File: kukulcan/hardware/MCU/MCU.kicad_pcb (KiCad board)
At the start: 4 copper layers, 90.1 x 64.4 mm, 90 parts, among them J1 Barrel_Jack_5V_In, J2 Barrel_Jack_5V_In, J3 USB_C_Receptacle, J4 SMA_GNSS, Q1 AO3401A, U1 TLV1117-33, U2 W25Q256JWEIQ, U3 ESP32-S3R16V, U4 BNO055, U5 NEO-M8N, U6 BMI088, U7 BME280, X1 40MHz, Y1 32.768kHz

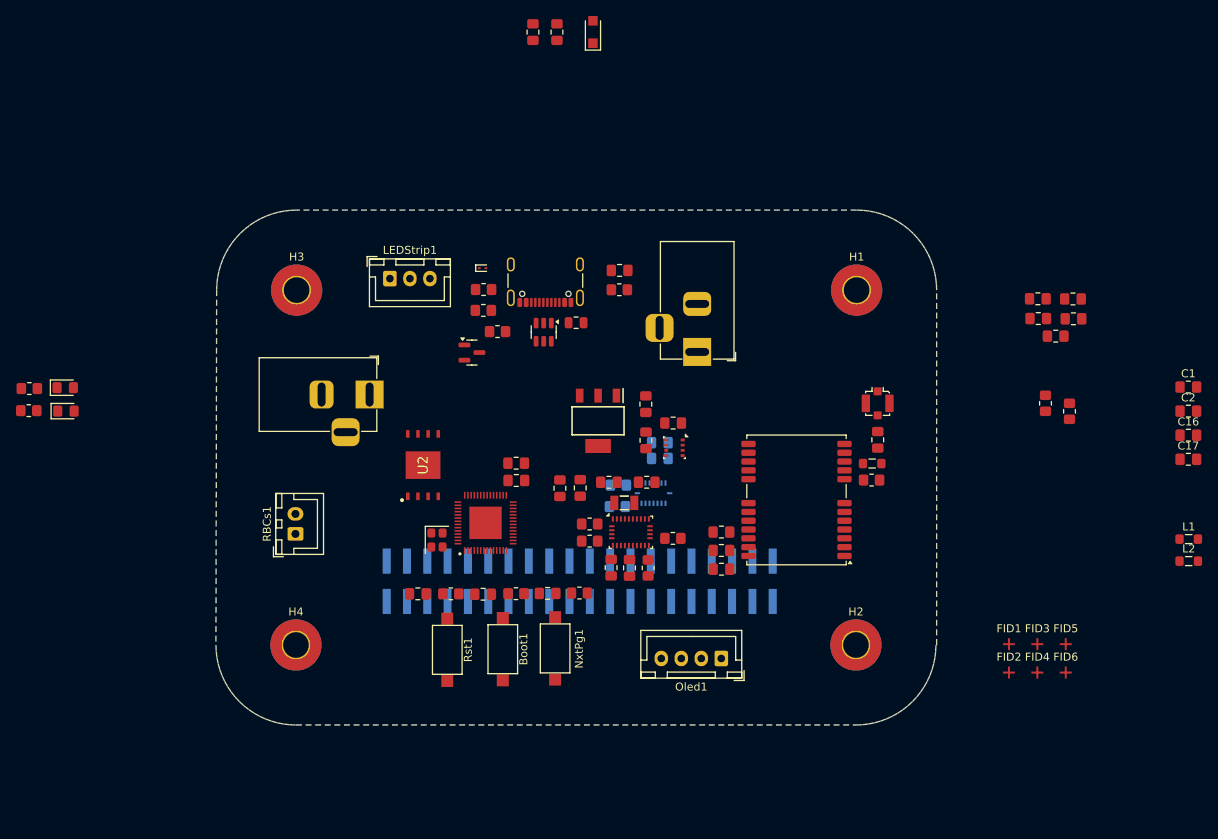
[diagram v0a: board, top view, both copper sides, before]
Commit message: feat(kukulcan): partial final PCB draft, GNSS pending
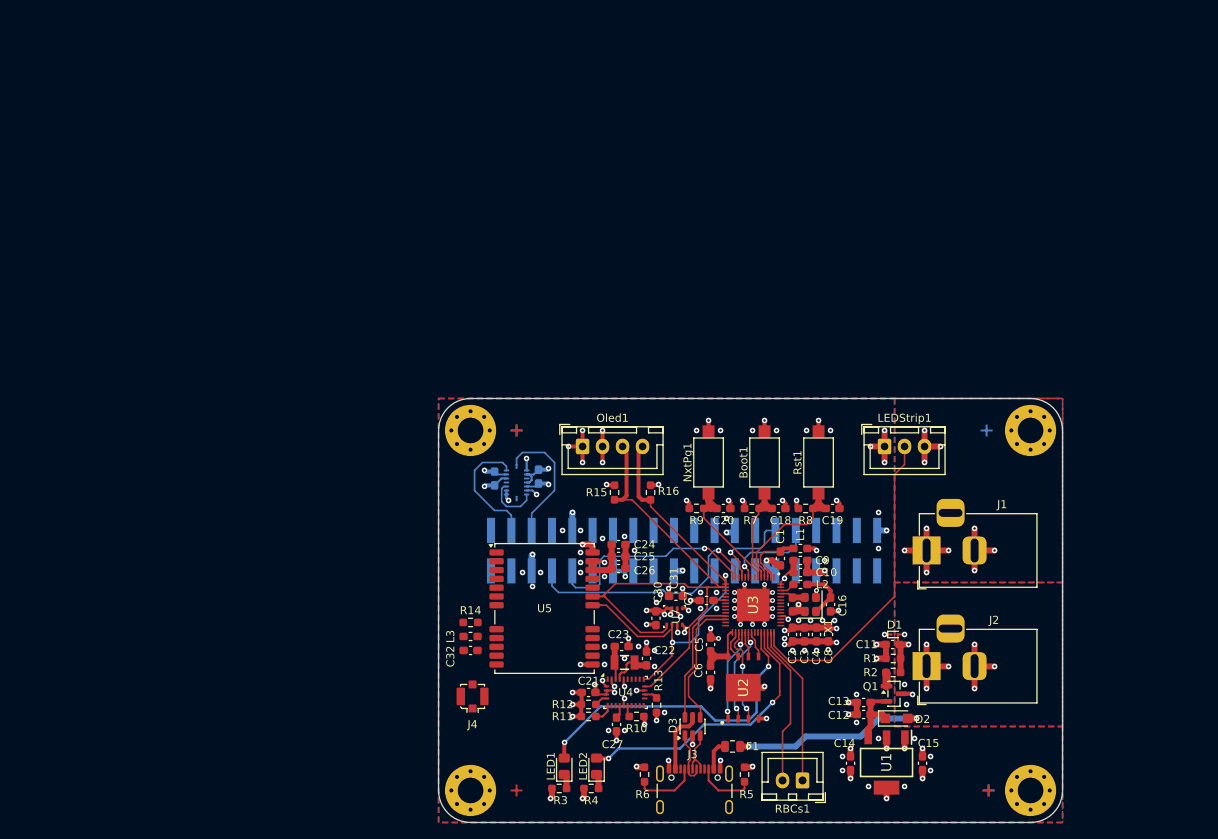
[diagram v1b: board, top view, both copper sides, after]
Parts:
- removed R17, R18: 10k/5%, Resistor_SMD:R_0805_2012Metric_Pad1.20x1.40mm_HandSolder
- C1, C10, C11, C12, C13, C14, C15, C16, C17, C18, C19, C2, C20, C21, C22, C23, C24, C25, C26, C27, C28, C29, C3, C30, C31, C32, C4, C5, C6, C7, C8, C9: footprint Capacitor_SMD:C_0805_2012Metric_Pad1.18x1.45mm_HandSolder -> Capacitor_SMD:C_0603_1608Metric_Pad1.08x0.95mm_HandSolder
- FID4, FID5, FID6: moved to B.Cu
- H1, H2, H3, H4: footprint MountingHole:MountingHole_3.2mm_M3_Pad_TopBottom -> MountingHole:MountingHole_3.2mm_M3_Pad_Via
- L1, L2, L3: footprint Inductor_SMD:L_0805_2012Metric_Pad1.05x1.20mm_HandSolder -> Inductor_SMD:L_0603_1608Metric_Pad1.05x0.95mm_HandSolder
- R1, R10, R13, R15, R2, R3, R4, R5, R6, R7, R8, R9: footprint Resistor_SMD:R_0805_2012Metric_Pad1.20x1.40mm_HandSolder -> Resistor_SMD:R_0603_1608Metric_Pad0.98x0.95mm_HandSolder
- R11, R12: value 5k1 -> 10k/5%; footprint Resistor_SMD:R_0805_2012Metric_Pad1.20x1.40mm_HandSolder -> Resistor_SMD:R_0603_1608Metric_Pad0.98x0.95mm_HandSolder
- R14: value 10k/5% -> 10R/1%; footprint Resistor_SMD:R_0805_2012Metric_Pad1.20x1.40mm_HandSolder -> Resistor_SMD:R_0603_1608Metric_Pad0.98x0.95mm_HandSolder
- R16: value 10R/1% -> 10k/5%; footprint Resistor_SMD:R_0805_2012Metric_Pad1.20x1.40mm_HandSolder -> Resistor_SMD:R_0603_1608Metric_Pad0.98x0.95mm_HandSolder
- moved C12 94.8 mm to (169.1, 117.5), turned to 180 degrees
- moved D2 93.8 mm to (173.2, 118.0), turned to 0 degrees
- moved C13 92.2 mm to (169.1, 116.0), turned to 180 degrees
- moved R4 84.7 mm to (135.1, 126.8)
- moved R3 83.0 mm to (131.1, 126.8)
- moved LED2 79.8 mm to (135.8, 124.0), turned to 90 degrees
- moved LED1 78.3 mm to (131.7, 124.0), turned to 90 degrees
- moved J1 72.3 mm to (177.0, 97.0), turned to 180 degrees
- moved FID4 71.8 mm to (125.8, 82.0), turned to 180 degrees
- moved RBCs1 70.5 mm to (161.5, 125.8), turned to 180 degrees
- moved R12 70.4 mm to (134.8, 116.2), turned to 0 degrees
- moved R11 69.2 mm to (134.8, 117.8), turned to 0 degrees
- moved D1 68.9 mm to (173.0, 107.5)
- moved J3 68.3 mm to (148.0, 128.0), turned to 0 degrees
- moved Q1 67.8 mm to (172.9, 114.9)
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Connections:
- J3 pad A1: (no net) -> GND
- J3 pad A12: (no net) -> GND
- J3 pad A4: (no net) -> +VUSB
- J3 pad A9: (no net) -> +VUSB
- J3 pad B1: (no net) -> GND
- J3 pad B12: (no net) -> GND
- J3 pad B4: (no net) -> +VUSB
- J3 pad B9: (no net) -> +VUSB
- Jetson1 pad 27: SDA -> unconnected-(Jetson1-Pin_27-Pad27)
- Jetson1 pad 28: SCL -> unconnected-(Jetson1-Pin_28-Pad28)
- Jetson1 pad 29: JT_MCU2 -> JT_MCU1
- Jetson1 pad 31: JT_MCU3 -> JT_MCU2
- Jetson1 pad 7: JT_MCU1 -> unconnected-(Jetson1-Pin_7-Pad7)
- LEDStrip1 pad 2: LedStripGPIO -> LedStrip
- R11 pad 1: +3V3 -> GND
- R11 pad 2: SDA -> Net-(U4-PS0)
- R12 pad 1: +3V3 -> GND
- R12 pad 2: SCL -> Net-(U4-PS1)
- R13 pad 2: Net-(U4-PS0) -> Net-(U4-COM3)
- R14 pad 1: GND -> Net-(U5-VCC_RF)
- R14 pad 2: Net-(U4-PS1) -> Net-(L3-Pad1)
- R15 pad 1: GND -> SCL
- R15 pad 2: Net-(U4-COM3) -> +3V3
- R16 pad 1: Net-(U5-VCC_RF) -> SDA
- R16 pad 2: Net-(L3-Pad1) -> +3V3
- U2 pad 9: (no net) -> GND
- U3 pad 11: unconnected-(U3-GPIO6-Pad11) -> JT_MCU1
- U3 pad 13: unconnected-(U3-GPIO8-Pad13) -> JT_TX
- U3 pad 14: unconnected-(U3-GPIO9-Pad14) -> JT_RX
- U3 pad 15: unconnected-(U3-GPIO10-Pad15) -> SDA
- U3 pad 16: unconnected-(U3-GPIO11-Pad16) -> SCL
- U3 pad 18: SDA -> unconnected-(U3-GPIO13-Pad18)
- U3 pad 19: SCL -> unconnected-(U3-GPIO14-Pad19)
- U3 pad 38: JT_MCU1 -> LED_WHITE
- U3 pad 39: JT_MCU2 -> LED_RED
- U3 pad 40: JT_MCU3 -> RB_TX
- U3 pad 41: LED_RED -> RB_RX
- U3 pad 42: LED_WHITE -> LedStrip
- U3 pad 43: LedStripGPIO -> unconnected-(U3-GPIO38-Pad43)
- U3 pad 47: RB_TX -> unconnected-(U3-MTDI-Pad47)
- U3 pad 48: RB_RX -> unconnected-(U3-MTMS-Pad48)
- U3 pad 8: JT_TX -> unconnected-(U3-GPIO3-Pad8)
- U3 pad 9: JT_RX -> JT_MCU2
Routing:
- net GND: track 0.00 -> 167.8 mm, vias 0 -> 124
- net SCL: track 0.00 -> 88.6 mm
- net SDA: track 0.00 -> 74.3 mm, vias 0 -> 2
- net +3V3: track 0.00 -> 61.9 mm, vias 0 -> 48
- net +VDD_5V: track 0.00 -> 41.2 mm, vias 0 -> 10
- net LedStrip: track 0.00 -> 40.1 mm
- net LED_WHITE: track 0.00 -> 40.0 mm, vias 0 -> 2
- net LED_RED: track 0.00 -> 34.8 mm, vias 0 -> 2
- net JT_TX: track 0.00 -> 31.4 mm, vias 0 -> 1
- net JT_RX: track 0.00 -> 27.5 mm, vias 0 -> 1
- net RB_RX: track 0.00 -> 20.1 mm
- net RB_TX: track 0.00 -> 20.1 mm
- net +RB_VDD_5V: track 0.00 -> 19.1 mm, vias 0 -> 7
- net RST: track 0.00 -> 18.4 mm
- net NxtPg: track 0.00 -> 16.4 mm
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- added copper zone on B.Cu, net +3V3
- added copper zone on F.Cu, net +3V3
- added copper zone on B.Cu, net +RB_VDD_5V
- added copper zone on F.Cu, net +RB_VDD_5V
- added copper zone on B.Cu, net +VDD_5V
- added copper zone on F.Cu, net +VDD_5V
- added copper zone on B.Cu, net GND
- added copper zone on F.Cu, net GND
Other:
- board size 90.1 x 64.4 mm -> 78 x 53 mm
